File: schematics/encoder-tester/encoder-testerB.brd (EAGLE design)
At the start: 121.9 x 45.4 mm, 17 parts, among them J3 POWER_JACKPTH_LOCK

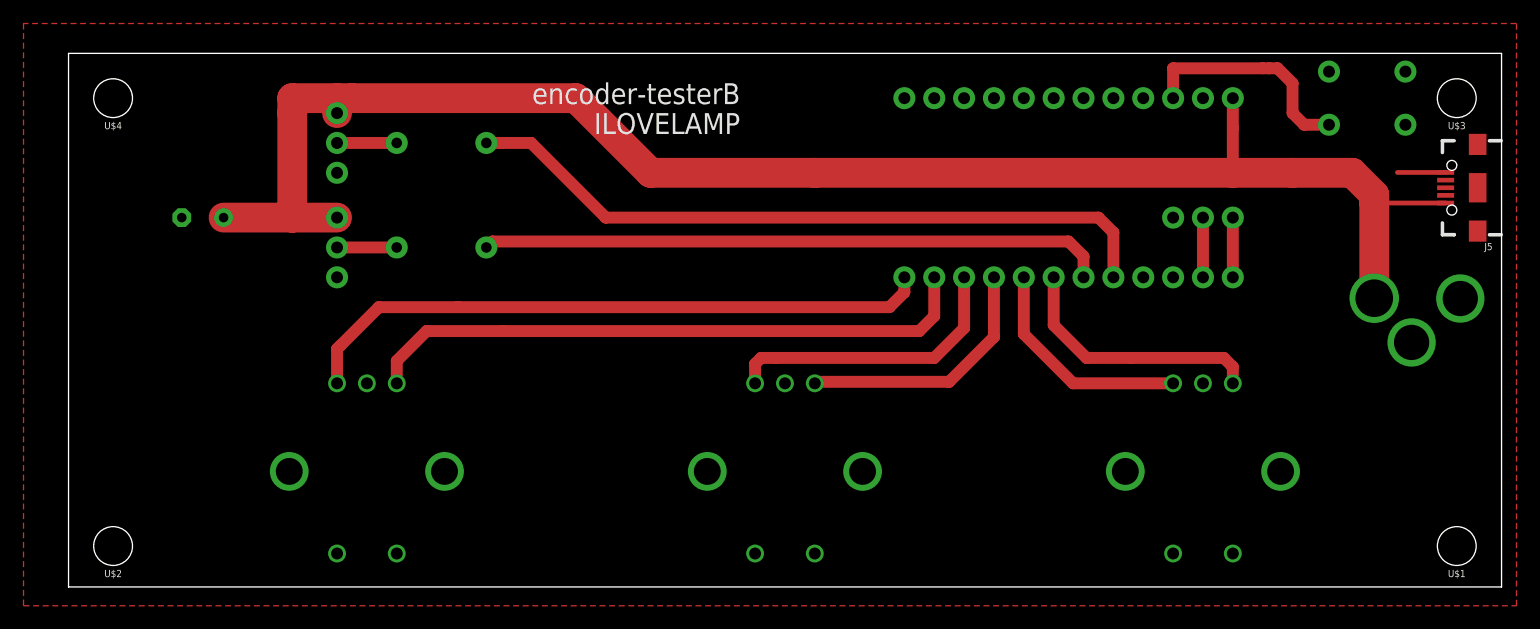
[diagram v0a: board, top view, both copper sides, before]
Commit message: small fixes
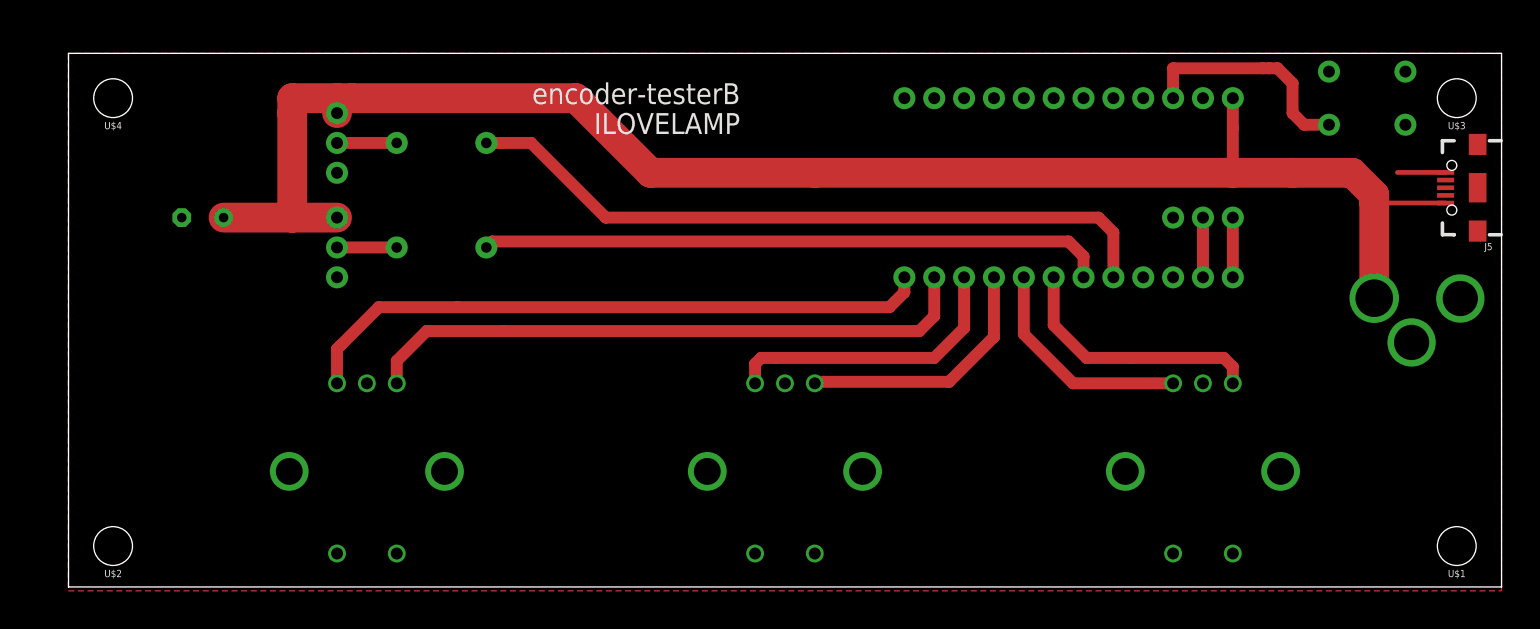
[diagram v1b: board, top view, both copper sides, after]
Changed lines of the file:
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@@
 <wire x1="121.92" y1="0.33" x2="121.92" y2="45.72" width="0" layer="20"/>
 <wire x1="125.73" y1="20.574" x2="-3.81" y2="20.574" width="0" layer="48" style="dashdot"/>
-<wire x1="60.96" y1="-5.08" x2="60.96" y2="69.85" width="0" layer="48" style="dashdot"/>
+<wire x1="60.96" y1="-5.08" x2="60.96" y2="49.53" width="0" layer="48" style="dashdot"/>
 <wire x1="124.714" y1="30.48" x2="-3.556" y2="30.48" width="0" layer="48" style="dashdot"/>
 <circle x="96.266" y="10.16" radius="14.02760625" width="0.0254" layer="48"/>
@@
 <contactref element="J2" pad="3"/>
 <polygon width="1.016" layer="1">
-<vertex x="-3.81" y="-1.27"/>
-<vertex x="123.19" y="-1.27"/>
-<vertex x="123.19" y="48.26"/>
-<vertex x="-3.81" y="48.26"/>
+<vertex x="0" y="0"/>
+<vertex x="121.92" y="0"/>
+<vertex x="121.92" y="45.72"/>
+<vertex x="0" y="45.72"/>
 </polygon>
 <contactref element="S4" pad="3"/>
@@
 <wire x1="117.163" y1="35.59" x2="113.06" y2="35.59" width="0.4064" layer="1"/>
 <wire x1="113.06" y1="35.59" x2="113.03" y2="35.56" width="0.254" layer="1"/>
+<wire x1="117.163" y1="35.59" x2="118.411" y2="24.8666" width="0" layer="19" extent="1-1"/>
 </signal>
 <signal name="ENC1A">
